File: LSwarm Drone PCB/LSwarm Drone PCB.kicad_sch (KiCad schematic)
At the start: 42 parts, among them J1 Conn_01x04_Pin, J2 USB_C_Receptacle_USB2.0_16P, U1 RP2350A, U3 LD1117V, U4 W25Q128JVS, Y1 12MHz

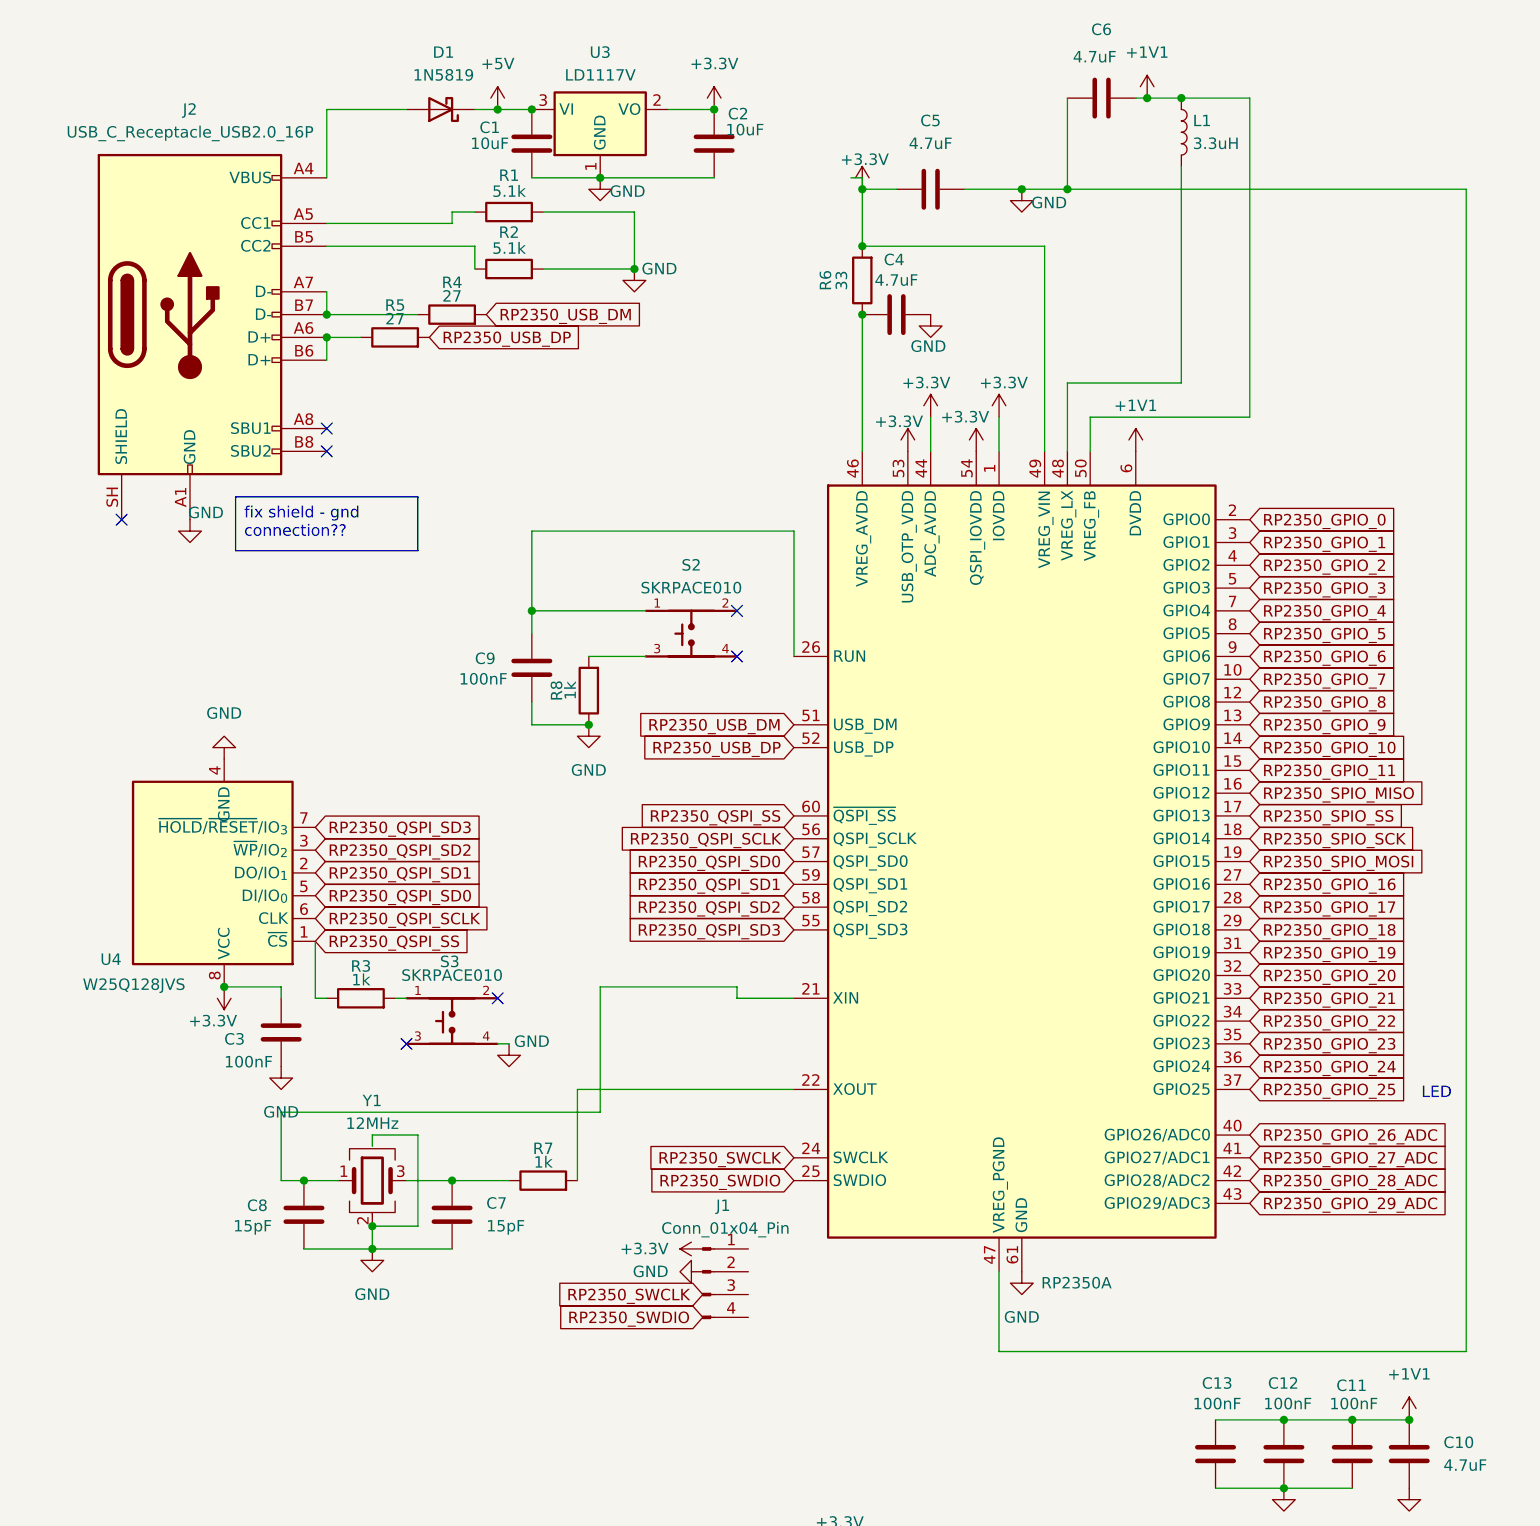
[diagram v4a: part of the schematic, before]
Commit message: sync
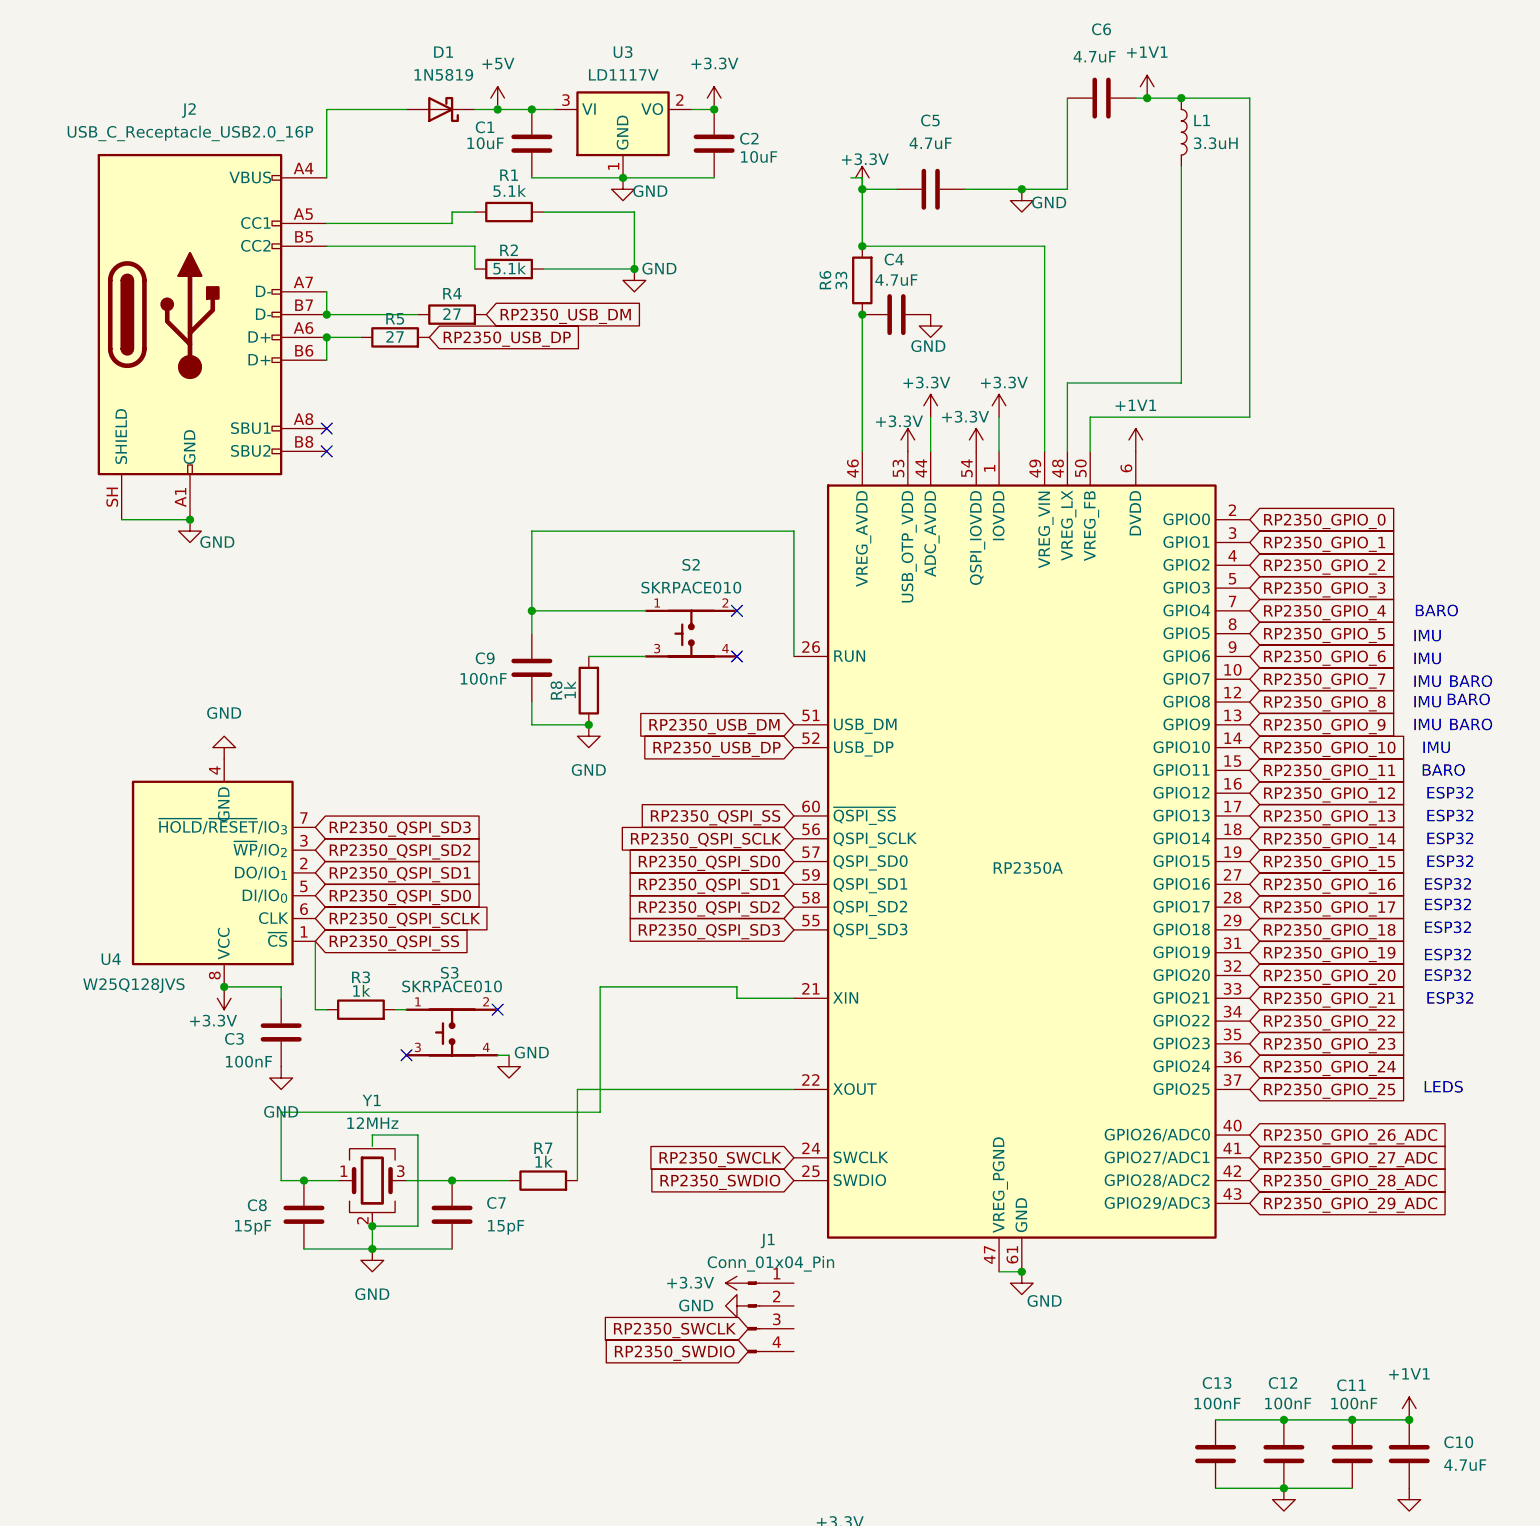
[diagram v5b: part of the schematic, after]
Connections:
- net GND: now also J2.SH (SHIELD)
- net RP2350_SPIO_MISO renamed RP2350_GPIO_12
- net RP2350_SPIO_MOSI renamed RP2350_GPIO_15
- net RP2350_SPIO_SCK renamed RP2350_GPIO_14
- net RP2350_SPIO_SS renamed RP2350_GPIO_13
- no-connect marks 7 -> 6
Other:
- note added: "BARO"
- note added: "ESP32"
- note added: "IMU"
- note added: "LEDS"
- note removed: "LED"
- moved on the sheet: J1, R3, S3, U3

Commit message: sync
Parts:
- added ANT2: ANT3216LL00R2400A, ANT3216LL00R2400A:ANTC3216X135N, symbol ANT3216LL00R2400A:ANT3216LL00R2400A
- added C38, C39, C40, C44, C46, C47, C48, C49, C50, C51, C53, C56, C57, C58: 100nF, symbol Device:C
- added C41, C59: 1uF, symbol Device:C
- added C42, C45: 10uF, symbol Device:C
- added C43: 22uF, symbol Device:C
- added C52, C55: 12pF, symbol Device:C
- added C54: 10nF, symbol Device:C
- added C60, C61: 3.3pF, symbol Device:C
- added J3: JST / BT2.0 Connector, Connector_JST:JST_PH_S2B-PH-K_1x02_P2.00mm_Horizontal, symbol Connector:Conn_01x02_Socket
- added L5: 2.2uH, symbol Device:L
- added L6: L, symbol Device:L
- added L7: 2nH, symbol Device:L
- added L8: 2.2nH, symbol Device:L
- added R14, R15, R16: 10k, symbol Device:R
- added R9: 470, symbol Device:R
- added S5, S6: SKRPACE010, SKRPACE010:SW_SKRPACE010, symbol SKRPACE010:SKRPACE010
- added U10: LSM6DSR, LSM6DSR:LGA-14L, symbol LSM6DSR:LSM6DSR
- added U11: BMP581, BMP581:BMP581, symbol BMP581:BMP581
- added U12: AP2112K-3.3, Package_TO_SOT_SMD:SOT-23-5, symbol Regulator_Linear:AP2112K-3.3
- added U13: TPS61023DRLR, TPS61023DRLR:SOT563-ORI, symbol TPS61023DRLR:TPS61023DRLR
- added U14: SN74LVC1T45DBVR, SN74LVC1T45DBVR:SOT95P280X145-6N, symbol SN74LVC1T45DBVR:SN74LVC1T45DBVR
- added U15, U16, U17, U18: SK6812MINI-E, symbol SK6812MINI-E:SK6812MINI-E
- added U6: ESP32-C3, Package_DFN_QFN:QFN-32-1EP_5x5mm_P0.5mm_EP3.7x3.7mm, symbol MCU_Espressif:ESP32-C3
- added Y3: 40MHz, symbol Device:Crystal_GND24
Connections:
- net +3.3V: now also C38.1, C39.2, C41.1, C53.1, C54.1, C56.1, C57.1, C58.1, L7.2, R14.1, R15.1, R16.1, U10.P$8 (VDD), U11.1 (VDDIO), U11.10 (VDD), U6.11 (VDD3P3_RTC), U6.17 (VDD3P3_CPU), U6.31 (VDDA), U6.32 (VDDA)
- net +5V: now also C43.2, C44.2, C46.2, C47.2, C48.2, L5.2, U13.6 (VOUT), U15.P$2 (VDD), U16.P$2 (VDD), U17.P$2 (VDD), U18.P$2 (VDD)
- net GND: now also C38.2, C40.2, C42.2, C43.1, C45.1, C46.1, C47.1, C48.1, C49.2, C50.2, C51.2, C52.2, C53.2, C54.2, C55.2, C56.2, C57.2, C58.2, C59.2, C60.2, C61.2, J3.2 (Pin_2), S5.4, S6.4, U10.P$2 (SDX), U10.P$3 (SCX), U10.P$6 (GND), U10.P$7 (GND), U11.3 (GND), U11.8 (GND), U11.9 (GND), U13.4 (GND), U15.P$1 (GND), U16.P$1 (GND), U17.P$1 (GND), U18.P$1 (GND), U6.33 (GND), Y3.2 (G), Y3.4 (G)
- net RP2350_GPIO_10: now also U10.P$12 (CS)
- net RP2350_GPIO_11: now also U11.6 (CSB)
- net RP2350_GPIO_12: now also U6.6 (GPIO2)
- net RP2350_GPIO_13: now also U6.16 (GPIO10)
- net RP2350_GPIO_14: now also C49.1, R15.2, S5.1, U6.7 (CHIP_EN)
- net RP2350_GPIO_15: now also C50.1, R16.2, S6.1, U6.15 (GPIO9)
- net RP2350_GPIO_16: now also U6.27 (U0RXD)
- net RP2350_GPIO_17: now also U6.28 (U0TXD)
- net RP2350_GPIO_25: now also R9.2
- net RP2350_GPIO_4: now also U11.7 (INT)
- net RP2350_GPIO_5: now also U10.P$4 (INT1)
- net RP2350_GPIO_6: now also U10.P$9 (INT2)
- net RP2350_GPIO_7: now also U10.P$13 (SCL), U11.2 (SCK/SCL)
- net RP2350_GPIO_8: now also U10.P$14 (SDA), U11.4 (SDI/SDA)
- net RP2350_GPIO_9: now also U10.P$1 (SDO), U11.5 (SDO/ADR)
- net RP2350_XIN: now reaches C8.1, U1.21 (XIN), Y1.1
- net RP2350_XOUT: now reaches R7.2, U1.22 (XOUT)
- new net: C44.1, C45.2
- new net: C60.1, L8.1, U6.1 (LNA_IN)
- new net: U16.P$4 (DOUT), U17.P$3 (DIN)
- new net: U17.P$4 (DOUT), U18.P$3 (DIN)
- new net: C52.1, L6.2, Y3.1
- new net: U15.P$4 (DOUT), U16.P$3 (DIN)
- new net: U10.P$10 (UNCONNECTED), U10.P$11 (UNCONNECTED)
- new net: C39.1, U10.P$5 (VDDIO)
- new net: L5.1, U13.5 (SW)
- new net: R9.1, U15.P$3 (DIN)
- new net: ANT2.1 (FEED), C61.1, L8.2
- new net: C40.1, C41.2
- new net BATT+: C42.1, J3.1 (Pin_1), U13.2 (EN), U13.3 (VIN)
- new net ESP32_40M_X0: L6.1, U6.30 (XTAL_P)
- new net ESP32_40M_X1: C55.1, U6.29 (XTAL_N), Y3.3
- new net ESP32_GPIO_0: U6.4 (XTAL_32K_P)
- new net ESP32_GPIO_1: U6.5 (XTAL_32K_N)
- new net ESP32_GPIO_18: U6.25 (GPIO18)
- new net ESP32_GPIO_19: U6.26 (GPIO19)
- new net ESP32_GPIO_3: U6.8 (GPIO3)
- new net ESP32_GPIO_8: R14.2, U6.14 (GPIO8)
- new net ESP32_VDD_3P3: C51.1, L7.1, U6.2 (VDD3P3), U6.3 (VDD3P3)
- new net ESP32_VDD_SPI: C59.1, U6.18 (VDD_SPI)
- no-connect marks 6 -> 21
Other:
- note added: "3.7v"
- note added: "BATTERY"
- note added: "ESP32 BOOT"
- note added: "ESP32 CRYSTAL"
- note added: "ESP32 EN"
- note added: "ESP32 VDD"
- note added: "FLASH RAM"
- note added: "GND"
- note added: "Near VDD & VDDA Pins"
- note added: "Near VDD_3P3"
- note added: "RP2350"
- note added: "RP2350 CRYSTAL"
- note added: "RP2350 DEBUG"
- note added: "USB-C Connector"
- moved on the sheet: C1, C10, C11, C12, C13, C14, C15, C16, C17, C18, C19, C2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

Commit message: sync
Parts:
- removed C1, C2: 10uF, symbol Device:C
- removed D1: 1N5819, Diode_THT:D_DO-41_SOD81_P10.16mm_Horizontal, symbol Diode:1N5819
- removed U3: LD1117V, Package_TO_SOT_THT:TO-220-3_Vertical, symbol Regulator_Linear:LD1117V
- added C25: 10nF, symbol Device:C
- added C62, C64, C66, C67, C68: 100nF, symbol Device:C
- added C63: 10uF, symbol Device:C
- added C65: 1uF, symbol Device:C
- added D1, D2, D3, D4: SS14, Diode_SMD:D_SMA, symbol Diode:SS14
- added J4, J5, J6, J7: Conn_01x02_Pin, symbol Connector:Conn_01x02_Pin
- added Q1, Q2, Q3, Q4: AO3400A, Package_TO_SOT_SMD:SOT-23, symbol Transistor_FET:AO3400A
- added R10, R19: 470, symbol Device:R
- added R11, R20, R22, R24: 10k, symbol Device:R
- added R12, R13, R21, R23: 100, symbol Device:R
- added R17: 806k, symbol Device:R
- added R18: 110k, symbol Device:R
- added U19: SK6812MINI-E, symbol SK6812MINI-E:SK6812MINI-E
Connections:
- net +3.3V: now also C39.1, U10.P$5 (VDDIO), U12.5 (VOUT), U14.1 (VCCA), U14.5 (DIR), C62.2, C64.2, C66.2, C68.1, U19.P$2 (VDD); no longer C39.2
- net +5V: now also U14.6 (VCCB), C67.2, R17.2
- net BATT+: now also U12.1 (VIN), U12.3 (EN), C65.2, D1.1 (K), D2.1 (K), D3.1 (K), D4.1 (K), J4.1 (Pin_1), J5.1 (Pin_1), J6.1 (Pin_1), J7.1 (Pin_1)
- net GND: now also C39.2, C4.1, U12.2 (GND), U14.2 (GND), C25.1, C63.1, C64.1, C65.1, C66.1, C67.1, C68.2, Q1.2 (S), Q2.2 (S), Q3.2 (S), Q4.2 (S), R11.1, R18.2, R20.1, R22.1, R24.1, U19.P$1 (GND); no longer C4.2, J2.SH (SHIELD)
- net RP2350_GPIO_18: now also R12.1
- net RP2350_GPIO_19: now also R13.1
- net RP2350_GPIO_20: now also R21.1
- net RP2350_GPIO_21: now also R23.1
- net RP2350_GPIO_24: now also R10.2
- net RP2350_GPIO_25: now also U14.3 (A); no longer R9.2
- net at R6.1, U1.46 (VREG_AVDD): now also C4.2; no longer C4.1
- net at U13.1 (FB): now also R17.1, R18.1
- net at U14.4 (B): now also R19.1
- new net: D2.2 (A), J5.2 (Pin_2), Q2.3 (D)
- new net: C25.2, J2.SH (SHIELD)
- new net: Q2.1 (G), R13.2, R20.2
- new net: Q1.1 (G), R11.2, R12.2
- new net: Q3.1 (G), R21.2, R22.2
- new net: D3.2 (A), J6.2 (Pin_2), Q3.3 (D)
- new net: C62.1, C63.2
- new net: Q4.1 (G), R23.2, R24.2
- new net: D1.2 (A), J4.2 (Pin_2), Q1.3 (D)
- new net: R10.1, U19.P$3 (DIN)
- new net: D4.2 (A), J7.2 (Pin_2), Q4.3 (D)
- new net RP2350_GPIO_25_5.5V: R19.2, R9.2
- no-connect marks 21 -> 22
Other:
- note added: "+"
- note added: "1.1V DECOUPLING"
- note added: "3.3V DECOUPLING"
- note added: "3.3V REG"
- note added: "3.3V-5V BOOST"
- note added: "3.3V-5V SIGNAL"
- note added: "ESP32-C3"
- note added: "LED ARRAY"
- note added: "MOTOR 1"
- note added: "MOTOR 2"
- note added: "MOTOR 3"
- note added: "MOTOR 4"
- note added: "Motor 1"
- note added: "Motor 2"
- note added: "Motor 3"
- note added: "Motor 4"
- note added: "STATUS LED"
- note added: "Voltage"
- note removed: "LEDS"
- moved on the sheet: C38, C39, C4, C40, C41, C43, C44, C45, C46, C47, C48, C9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

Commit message: finished the schematic!!!!
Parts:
- added BUZZER1: MLT-5020, easyeda2kicad:BUZ-SMD_L5.0-W5.5-P4.60, symbol MLT-5020:MLT-5020
- added C71: 100nF, symbol Device:C
- added C71Ceramic1: 10uF, symbol Device:C
- added C72: 220uF, symbol Device:C
- added Q5: AO3401A, Package_TO_SOT_SMD:SOT-23, symbol Transistor_FET:AO3401A
- added R25, R26: 220k, symbol Device:R
- added R27: 100, symbol Device:R
- added R28: 100k, symbol Device:R
- added S1: MSK12C02, MSK12C02:SW_MSK12C02, symbol MSK12C02:MSK12C02
- R11, R20, R22, R24: value 10k -> 4.7k
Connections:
- net ESP32_VDD_SPI is gone; now on net +3.3V: C59.1, U6.18 (VDD_SPI)
- net BATT+: now also Q5.2 (S), R28.2; no longer C42.1, C65.2, D1.1 (K), D2.1 (K), D3.1 (K), D4.1 (K), J4.1 (Pin_1), J5.1 (Pin_1), J6.1 (Pin_1), J7.1 (Pin_1), U12.1 (VIN), U12.3 (EN), U13.2 (EN), U13.3 (VIN)
- net GND: now also BUZZER1.2 (-), C71.1, C71Ceramic1.1, C72.1, R26.1, S1.3
- net RP2350_GPIO_22: now also R27.1
- net RP2350_GPIO_26_ADC: now also C71.2, R25.2, R26.2
- net ESP32_GPIO_0: no longer names the net of U6.4 (XTAL_32K_P)
- net ESP32_GPIO_1: no longer names the net of U6.5 (XTAL_32K_N)
- net ESP32_GPIO_18: no longer names the net of U6.25 (GPIO18)
- net ESP32_GPIO_19: no longer names the net of U6.26 (GPIO19)
- net ESP32_GPIO_3: no longer names the net of U6.8 (GPIO3)
- net ESP32_GPIO_8: no longer names the net of R14.2, U6.14 (GPIO8)
- new net: BUZZER1.1 (+), R27.2
- new net: Q5.1 (G), R28.1, S1.2
- new net: S1.4_1 (GND), S1.4_2 (GND), S1.4_3 (GND), S1.4_4 (GND)
- new net BATT_SW+: C42.1, C65.2, C71Ceramic1.2, C72.2, D1.1 (K), D2.1 (K), D3.1 (K), D4.1 (K), J4.1 (Pin_1), J5.1 (Pin_1), J6.1 (Pin_1), J7.1 (Pin_1), Q5.3 (D), R25.1, U12.1 (VIN), U12.3 (EN), U13.2 (EN), U13.3 (VIN)
- no-connect marks 22 -> 30
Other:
- note added: "ARM"
- note added: "BUZZ"
- note added: "V MON"
- note removed: "Voltage"
- moved on the sheet: C62, C63, C64, C65, J3, R10, R14, U12, U19
